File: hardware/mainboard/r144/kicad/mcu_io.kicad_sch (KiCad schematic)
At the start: 47 parts, among them J2 Hirose DM3AT-SF-PEJM5, SW2 BOOT / RECOVERY, SW3 TL1016AAF160QG, SW4 TL1016AAF160QG, SW5 TL1016AAF160QG, SW6 TL1016AAF160QG, U1 ESP32-S3-WROOM-1-N16R8, U10 TLV3012BIDBVR, U11 TPS389001DSER, U5 BMI270, U9 TMUX1101DBVR

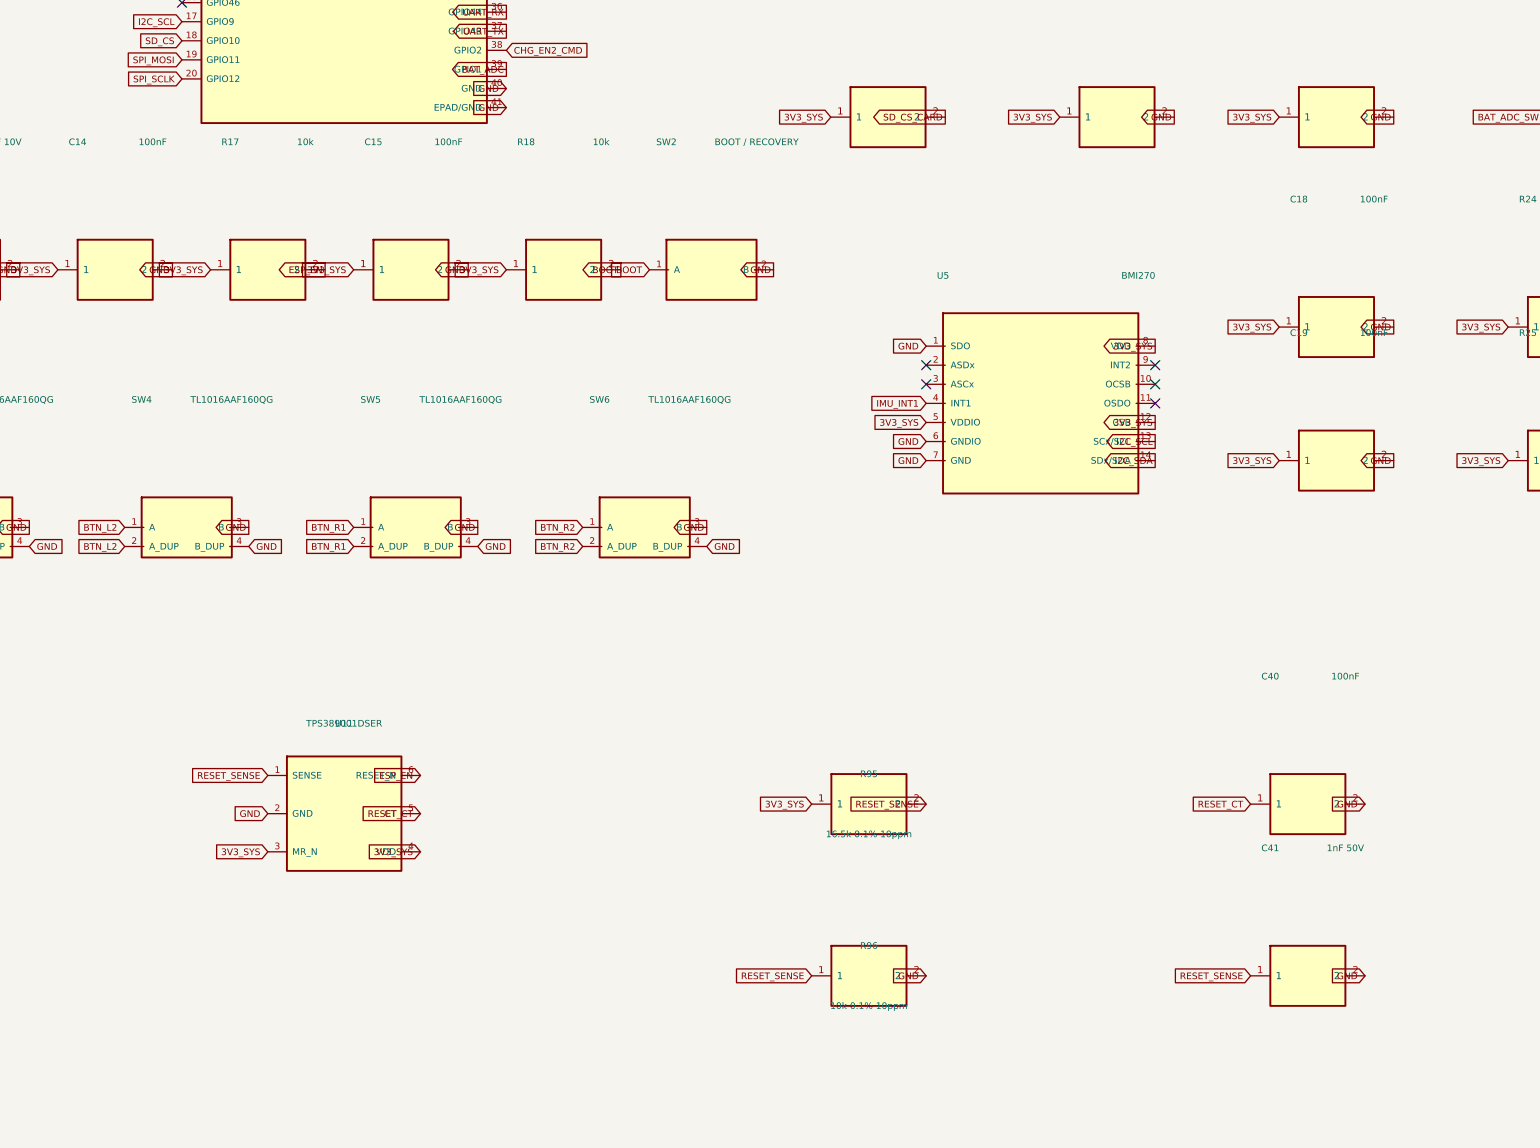
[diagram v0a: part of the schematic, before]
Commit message: hardware(r144): route precision reset and PWM supply, fix rule compilation; native checks zero, independent review pending
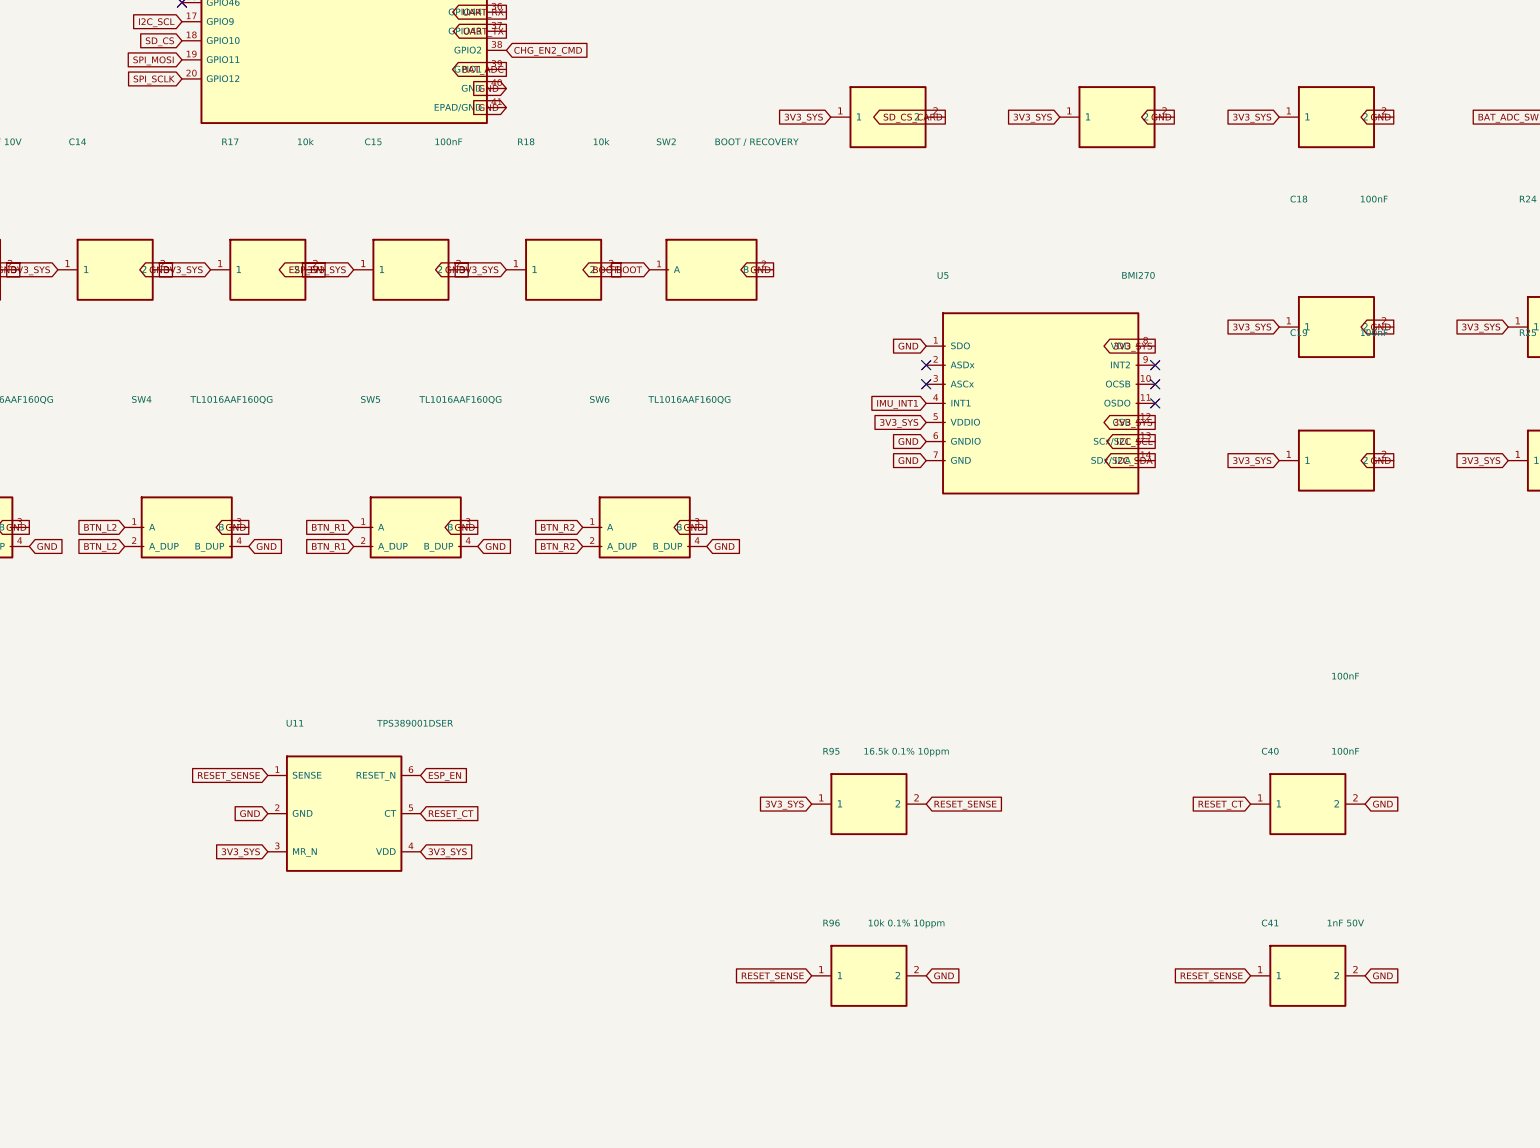
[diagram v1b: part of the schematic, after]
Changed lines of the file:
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@@
 	(symbol (lib_id "ENKU:C") (at 52.07 132.08 0) (unit 1) (exclude_from_sim no) (in_bom yes) (on_board yes) (dnp no)
 		(property "Reference" "C14" (at 47.07 115.08 0) (effects (font (size 0.88 0.88))))
-		(property "Value" "100nF" (at 57.07 115.08 0) (effects (font (size 0.88 0.88))))
+		(property "Value" "100nF" (at 215.820000 196.200000 0) (effects (font (size 0.88 0.88))))
 		(property "Footprint" "ENKU:C_CC0603_YAGEO_REFLOW_TRANSFER" (at 52.07 132.08 0) (effects (font (size 0.88 0.88)) (hide yes)))
 		(property "Datasheet" "https://yageogroup.com/download/specsheet/CC0603KRX7R9BB104" (at 52.07 132.08 0) (effects (font (size 0.88 0.88)) (hide yes)))
@@
 (global_label "GND" (shape input) (at 130.810000 168.910000 180) (effects (font (size .88 .88)) (justify left bottom)))
 (symbol (lib_id "ENKU:TPS3890") (at 82.55 204.47 0) (unit 1) (exclude_from_sim no) (in_bom yes) (on_board yes) (dnp no)
-(property "Reference" "U11" (at 82.55 192.47 0) (effects (font (size .88 .88))))
-(property "Value" "TPS389001DSER" (at 82.55 192.47 0) (effects (font (size .88 .88))))
+(property "Reference" "U11" (at 76 192.47 0) (effects (font (size .88 .88))))
+(property "Value" "TPS389001DSER" (at 92 192.47 0) (effects (font (size .88 .88))))
 (property "Footprint" "ENKU:TPS3890_TI_DSE0006A_SMD_LEFT" (at 82.55 204.47 0) (effects (font (size .88 .88)) (hide yes)))
 (property "Datasheet" "https://www.ti.com/lit/ds/symlink/tps3890.pdf" (at 82.55 204.47 0) (effects (font (size .88 .88)) (hide yes)))
@@
 (global_label "GND" (shape input) (at 72.390000 204.470000 0) (effects (font (size .88 .88)) (justify right bottom)))
 (global_label "3V3_SYS" (shape input) (at 72.390000 209.550000 0) (effects (font (size .88 .88)) (justify right bottom)))
-(global_label "3V3_SYS" (shape input) (at 92.710000 209.550000 0) (effects (font (size .88 .88)) (justify right bottom)))
-(global_label "RESET_CT" (shape input) (at 92.710000 204.470000 0) (effects (font (size .88 .88)) (justify right bottom)))
-(global_label "ESP_EN" (shape input) (at 92.710000 199.390000 0) (effects (font (size .88 .88)) (justify right bottom)))
+(global_label "3V3_SYS" (shape input) (at 92.710000 209.550000 180) (effects (font (size .88 .88)) (justify left bottom)))
+(global_label "RESET_CT" (shape input) (at 92.710000 204.470000 180) (effects (font (size .88 .88)) (justify left bottom)))
+(global_label "ESP_EN" (shape input) (at 92.710000 199.390000 180) (effects (font (size .88 .88)) (justify left bottom)))
 (symbol (lib_id "ENKU:R") (at 152.400000 203.200000 0) (unit 1) (exclude_from_sim no) (in_bom yes) (on_board yes) (dnp no)
-(property "Reference" "R95" (at 152.400000 199.200000 0) (effects (font (size .88 .88))))
-(property "Value" "16.5k 0.1% 10ppm" (at 152.400000 207.200000 0) (effects (font (size .88 .88))))
+(property "Reference" "R95" (at 147.400000 196.200000 0) (effects (font (size .88 .88))))
+(property "Value" "16.5k 0.1% 10ppm" (at 157.400000 196.200000 0) (effects (font (size .88 .88))))
 (property "Footprint" "ENKU:R_RT0603_YAGEO_REFLOW" (at 152.400000 203.200000 0) (effects (font (size .88 .88)) (hide yes)))
 (property "Datasheet" "https://yageogroup.com/content/datasheet/asset/file/PYU-RT_1-TO-0-01_ROHS_L" (at 152.400000 203.200000 0) (effects (font (size .88 .88)) (hide yes)))
@@
 )
 (global_label "3V3_SYS" (shape input) (at 144.780000 203.200000 0) (effects (font (size .88 .88)) (justify right bottom)))
-(global_label "RESET_SENSE" (shape input) (at 160.020000 203.200000 0) (effects (font (size .88 .88)) (justify right bottom)))
+(global_label "RESET_SENSE" (shape input) (at 160.020000 203.200000 180) (effects (font (size .88 .88)) (justify left bottom)))
 (symbol (lib_id "ENKU:R") (at 152.400000 226.060000 0) (unit 1) (exclude_from_sim no) (in_bom yes) (on_board yes) (dnp no)
-(property "Reference" "R96" (at 152.400000 222.060000 0) (effects (font (size .88 .88))))
-(property "Value" "10k 0.1% 10ppm" (at 152.400000 230.060000 0) (effects (font (size .88 .88))))
+(property "Reference" "R96" (at 147.400000 219.060000 0) (effects (font (size .88 .88))))
+(property "Value" "10k 0.1% 10ppm" (at 157.400000 219.060000 0) (effects (font (size .88 .88))))
 (property "Footprint" "ENKU:R_RT0603_YAGEO_REFLOW" (at 152.400000 226.060000 0) (effects (font (size .88 .88)) (hide yes)))
 (property "Datasheet" "https://yageogroup.com/content/datasheet/asset/file/PYU-RT_1-TO-0-01_ROHS_L" (at 152.400000 226.060000 0) (effects (font (size .88 .88)) (hide yes)))
@@
 )
 (global_label "RESET_SENSE" (shape input) (at 144.780000 226.060000 0) (effects (font (size .88 .88)) (justify right bottom)))
-(global_label "GND" (shape input) (at 160.020000 226.060000 0) (effects (font (size .88 .88)) (justify right bottom)))
+(global_label "GND" (shape input) (at 160.020000 226.060000 180) (effects (font (size .88 .88)) (justify left bottom)))
 (symbol (lib_id "ENKU:C") (at 210.820000 203.200000 0) (unit 1) (exclude_from_sim no) (in_bom yes) (on_board yes) (dnp no)
-		(property "Reference" "C40" (at 205.820000 186.200000 0) (effects (font (size 0.88 0.88))))
+		(property "Reference" "C40" (at 205.820000 196.200000 0) (effects (font (size 0.88 0.88))))
 		(property "Value" "100nF" (at 215.820000 186.200000 0) (effects (font (size 0.88 0.88))))
 		(property "Footprint" "ENKU:C_CC0603_YAGEO_REFLOW_TRANSFER" (at 210.820000 203.200000 0) (effects (font (size 0.88 0.88)) (hide yes)))
@@
 	)
 (global_label "RESET_CT" (shape input) (at 203.200000 203.200000 0) (effects (font (size .88 .88)) (justify right bottom)))
-(global_label "GND" (shape input) (at 218.440000 203.200000 0) (effects (font (size .88 .88)) (justify right bottom)))
+(global_label "GND" (shape input) (at 218.440000 203.200000 180) (effects (font (size .88 .88)) (justify left bottom)))
 (symbol (lib_id "ENKU:C") (at 210.820000 226.060000 0) (unit 1) (exclude_from_sim no) (in_bom yes) (on_board yes) (dnp no)
-		(property "Reference" "C41" (at 205.820000 209.060000 0) (effects (font (size 0.88 0.88))))
-		(property "Value" "1nF 50V" (at 215.820000 209.060000 0) (effects (font (size 0.88 0.88))))
+		(property "Reference" "C41" (at 205.820000 219.060000 0) (effects (font (size 0.88 0.88))))
+		(property "Value" "1nF 50V" (at 215.820000 219.060000 0) (effects (font (size 0.88 0.88))))
 		(property "Footprint" "ENKU:C_CC0603_YAGEO_REFLOW_TRANSFER" (at 210.820000 226.060000 0) (effects (font (size 0.88 0.88)) (hide yes)))
 		(property "Datasheet" "https://yageogroup.com/download/specsheet/CC0603JRNPO9BN102" (at 210.820000 226.060000 0) (effects (font (size 0.88 0.88)) (hide yes)))
@@
 	)
 (global_label "RESET_SENSE" (shape input) (at 203.200000 226.060000 0) (effects (font (size .88 .88)) (justify right bottom)))
-(global_label "GND" (shape input) (at 218.440000 226.060000 0) (effects (font (size .88 .88)) (justify right bottom)))
-)
+(global_label "GND" (shape input) (at 218.440000 226.060000 180) (effects (font (size .88 .88)) (justify left bottom)))
+)
